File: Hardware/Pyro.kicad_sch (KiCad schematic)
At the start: 33 parts, among them J12 Conn_01x02_Male, Q7 BSZ025N04LS, U10 SiC438BED-T1-GE3, U12 INA219AxDCN, U9 782-TCMT1109

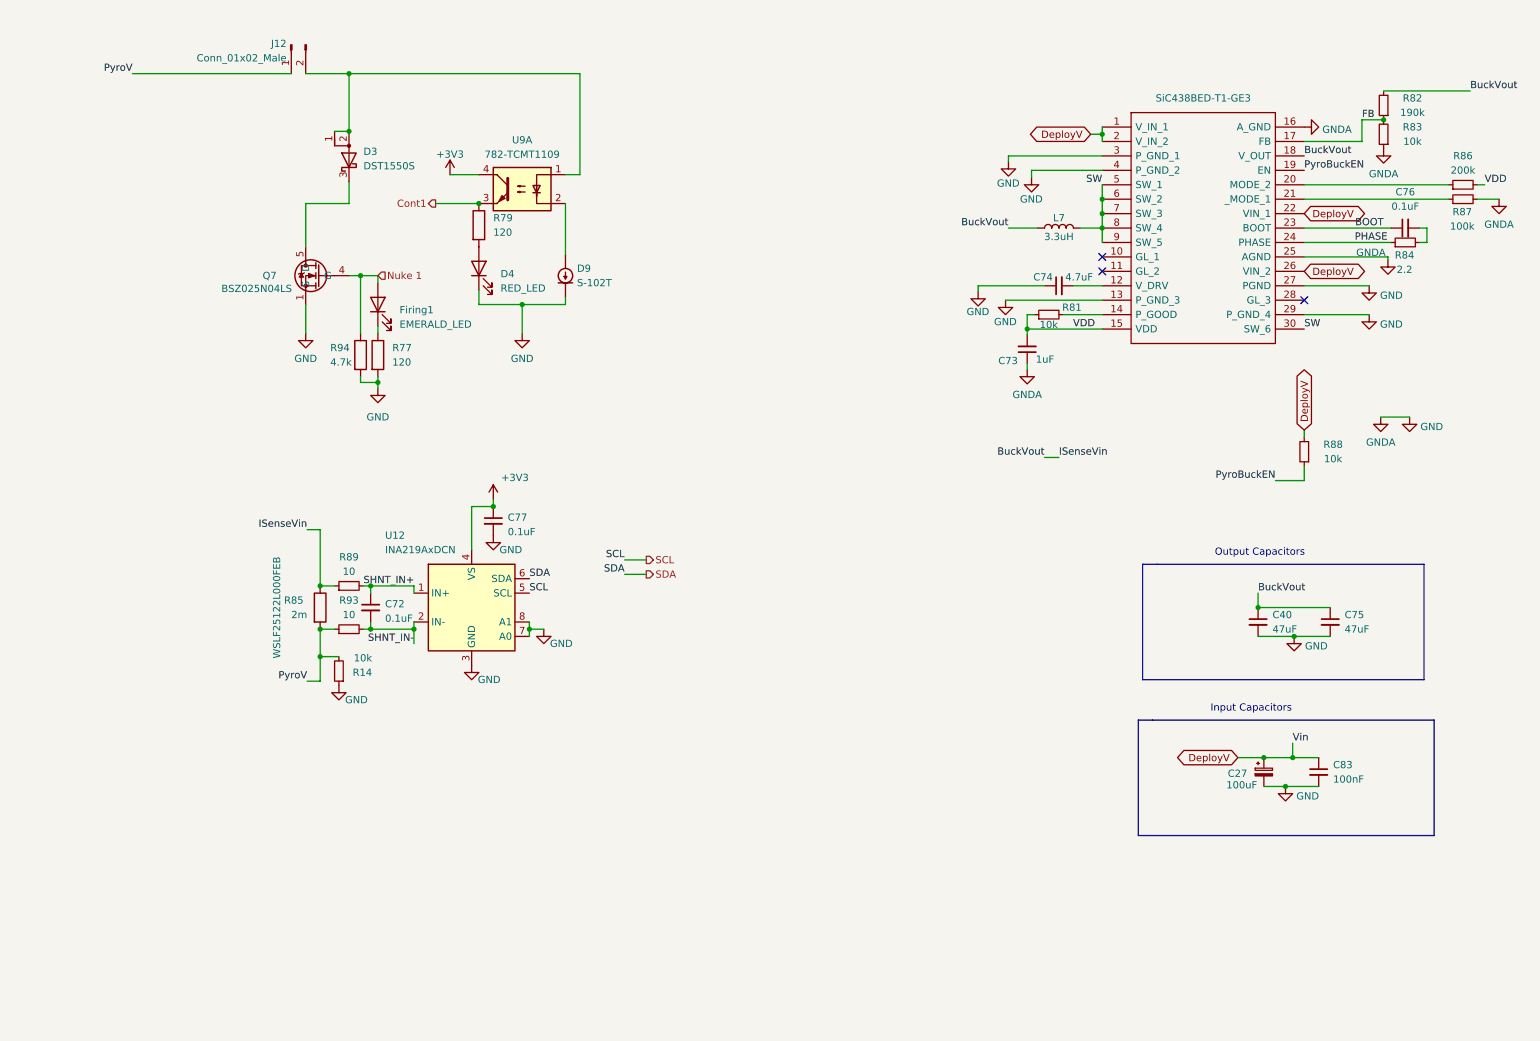
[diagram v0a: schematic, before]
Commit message: Solenoid Feature and minor changes
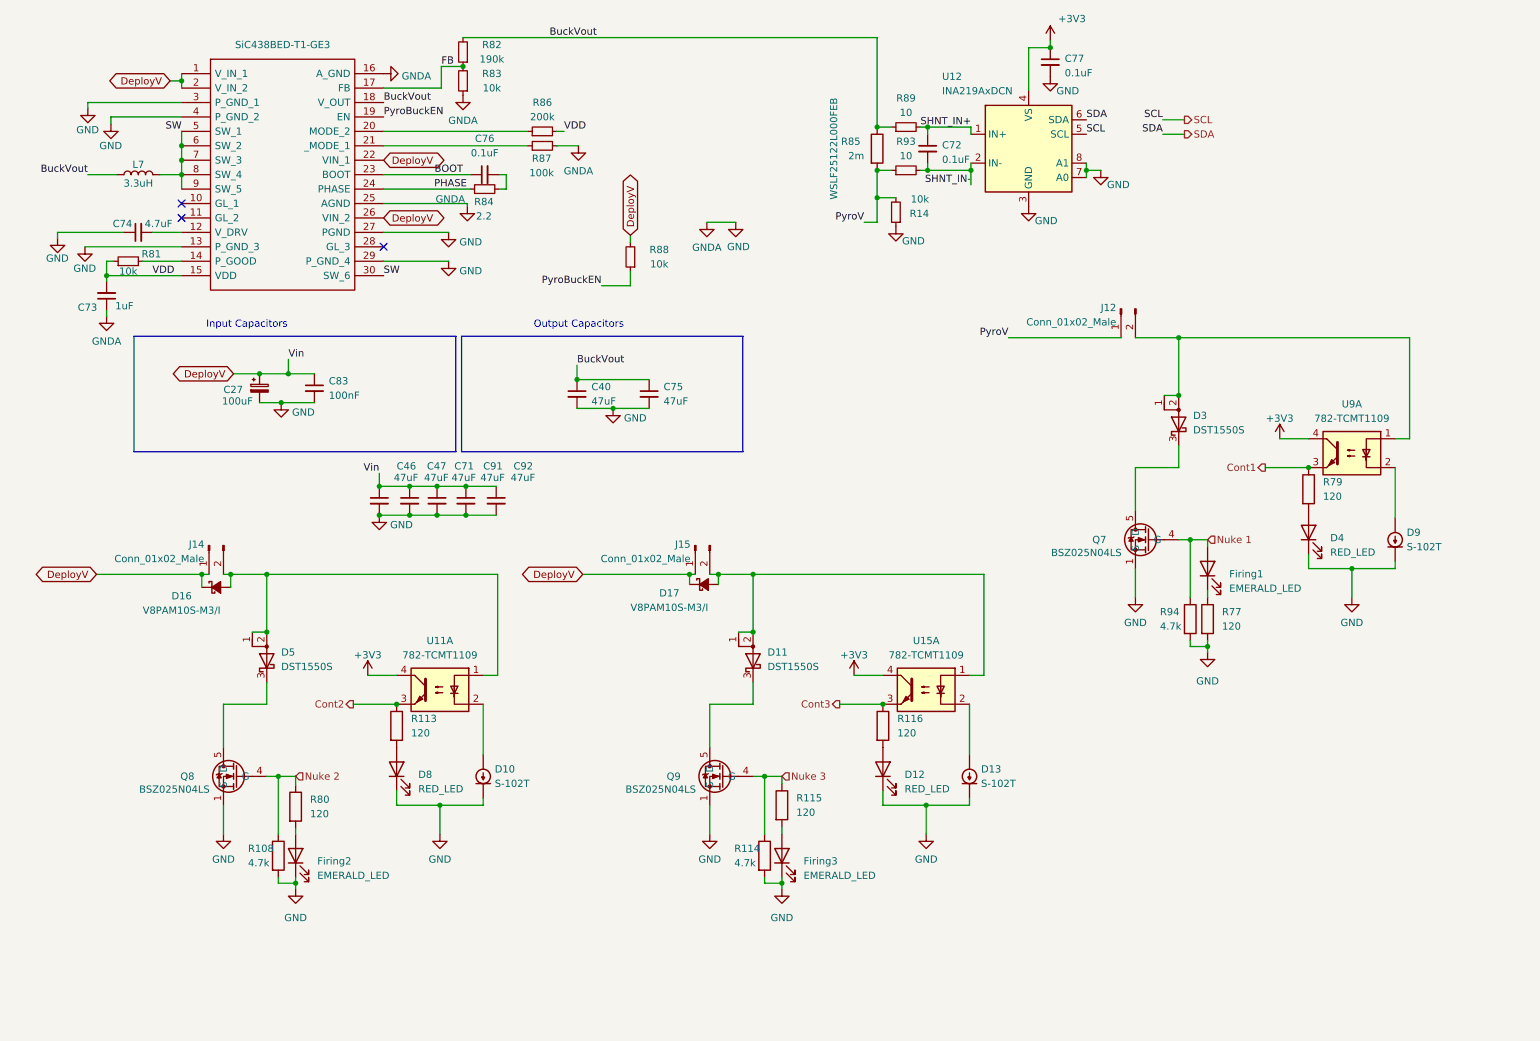
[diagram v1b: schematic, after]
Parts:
- added C46, C47, C71, C91, C92: 47uF, Capacitor_SMD:C_1206_3216Metric, symbol Device:C_Small
- added D10, D13: S-102T, iclr:SODFL3516X70N, symbol Device:D_Current-regulator
- added D11, D5: DST1550S, Package_TO_SOT_SMD:TO-277B, symbol Device:D_Schottky_AAK
- added D12, D8: RED_LED, LED_SMD:LED_0603_1608Metric, symbol Device:LED
- added D16, D17: V8PAM10S-M3/I, iclr:V8PAM10SM3I, symbol Device:D_Schottky_Small_Filled
- added Firing2, Firing3: EMERALD_LED, LED_SMD:LED_0402_1005Metric, symbol Device:LED
- added J14, J15: Conn_01x02_Male, Connector_Molex:Molex_Nano-Fit_105313-xx02_1x02_P2.50mm_Horizontal, symbol Connector:Conn_01x02_Male
- added Q8, Q9: BSZ025N04LS, iclr:BSZ025N04LS, symbol iclr:BSZ025N04LS
- added R108, R114: 4.7k, Resistor_SMD:R_0402_1005Metric, symbol Device:R
- added R113, R116: 120, Resistor_SMD:R_0603_1608Metric, symbol Device:R
- added R115, R80: 120, Resistor_SMD:R_0402_1005Metric, symbol Device:R
- added U11, U15: 782-TCMT1109, iclr:TCMT1109-4N, symbol Isolator:LTV-247
- R82: footprint Resistor_SMD:R_0402_1005Metric -> Resistor_SMD:R_0603_1608Metric_Pad0.98x0.95mm_HandSolder
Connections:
- net +3V3: now also U11.4, U15.4
- net DeployV: now also C46.1, C47.1, C71.1, C91.1, C92.1, D16.1 (K), D17.1 (K), J14.1 (Pin_1), J15.1 (Pin_1)
- net GND: now also C46.2, C47.2, C71.2, C91.2, C92.2, D10.1 (K), D12.1 (K), D13.1 (K), D8.1 (K), Firing2.1 (K), Firing3.1 (K), Q8.1 (S), Q8.2 (S), Q8.3 (S), Q8.A1 (S), Q9.1 (S), Q9.2 (S), Q9.3 (S), Q9.A1 (S), R108.2, R114.2
- new net: D8.2 (A), R113.2
- new net: D11.1 (A), D11.2 (A), D17.2 (A), J15.2 (Pin_2), U15.1
- new net: D11.3 (K), Q9.5 (D), Q9.6 (D), Q9.7 (D), Q9.8 (D), Q9.A5 (D)
- new net: D16.2 (A), D5.1 (A), D5.2 (A), J14.2 (Pin_2), U11.1
- new net: D10.2 (A), U11.2
- new net: D13.2 (A), U15.2
- new net: D5.3 (K), Q8.5 (D), Q8.6 (D), Q8.7 (D), Q8.8 (D), Q8.A5 (D)
- new net: Firing2.2 (A), R80.2
- new net: D12.2 (A), R116.2
- new net: Firing3.2 (A), R115.2
- new net Cont2: R113.1, U11.3
- new net Cont3: R116.1, U15.3
- new net Nuke 2: Q8.4 (G), R108.1, R80.1
- new net Nuke 3: Q9.4 (G), R114.1, R115.1
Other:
- moved on the sheet: C27, C40, C72, C73, C74, C75, C76, C77, C83, D3, D4, D9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

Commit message: Review Changes
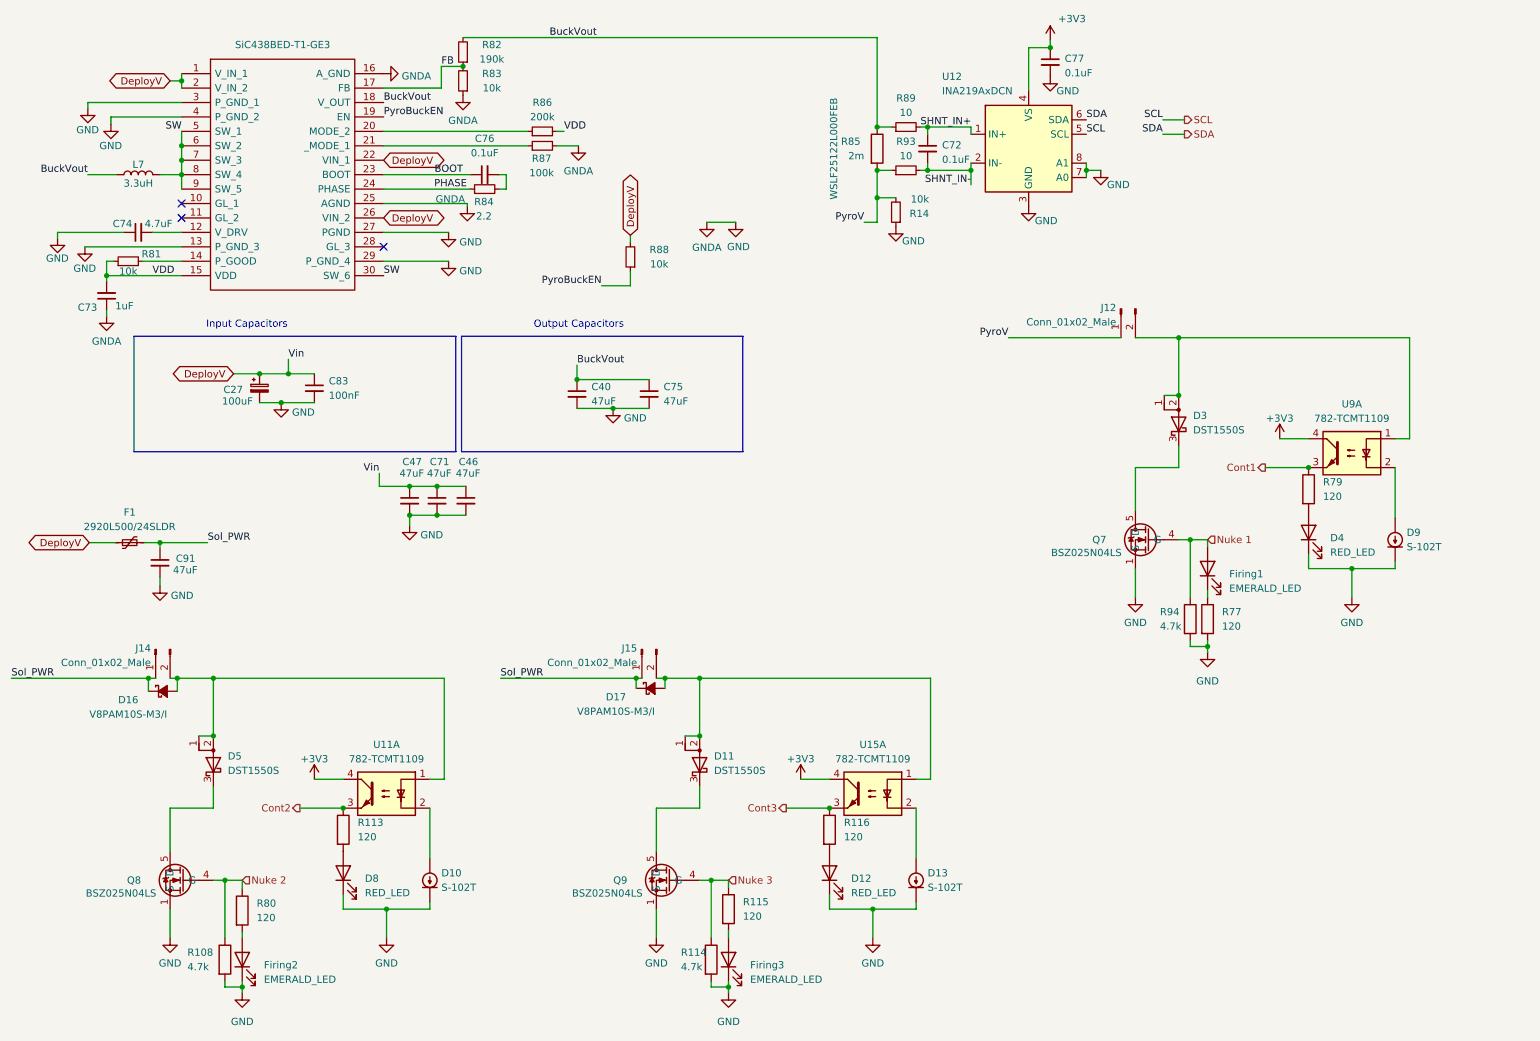
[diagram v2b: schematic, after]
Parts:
- removed C92: 47uF, Capacitor_SMD:C_1206_3216Metric, symbol Device:C_Small
- added F1: 2920L500/24SLDR, Fuse:Fuse_2920_7451Metric, symbol Device:Polyfuse_Small
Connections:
- net DeployV: now also F1.1; no longer C91.1, D16.1 (K), D17.1 (K), J14.1 (Pin_1), J15.1 (Pin_1)
- new net Sol_PWR: C91.1, D16.1 (K), D17.1 (K), F1.2, J14.1 (Pin_1), J15.1 (Pin_1)
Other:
- moved on the sheet: C46, C91, D10, D11, D12, D13, D16, D17, D5, D8, Firing2, Firing3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
